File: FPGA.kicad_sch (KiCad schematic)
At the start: 37 parts, among them U7 ICE40HX8K-CB132, X1 XO53

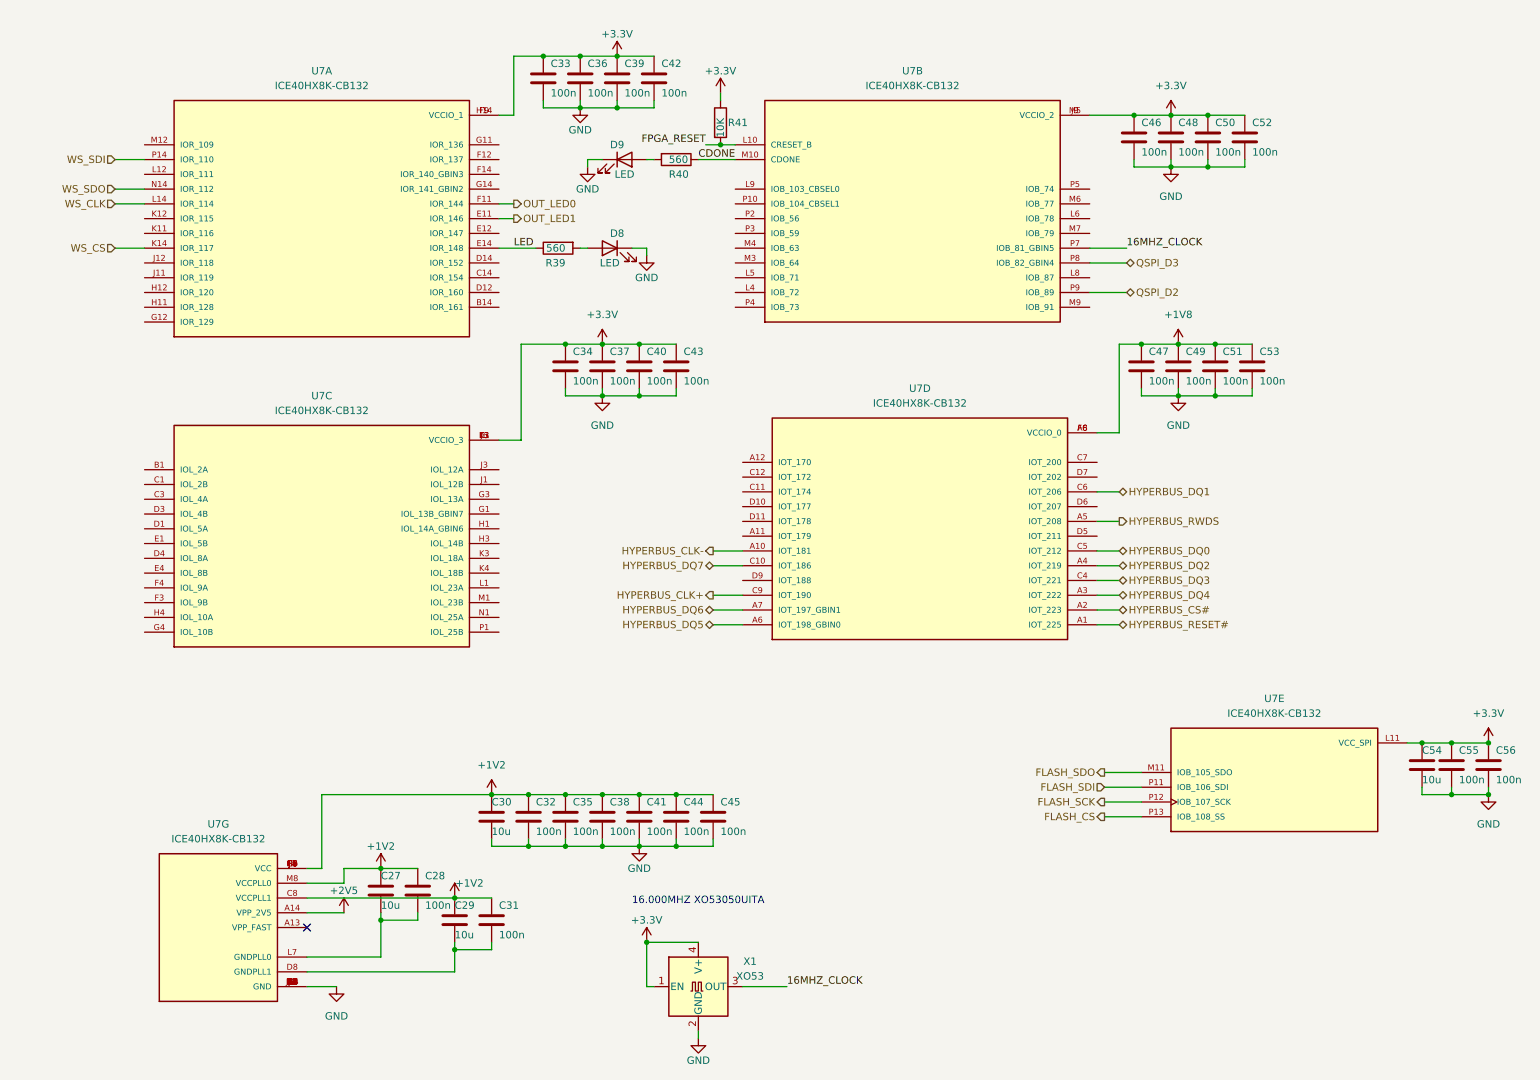
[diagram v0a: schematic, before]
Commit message: Start routing
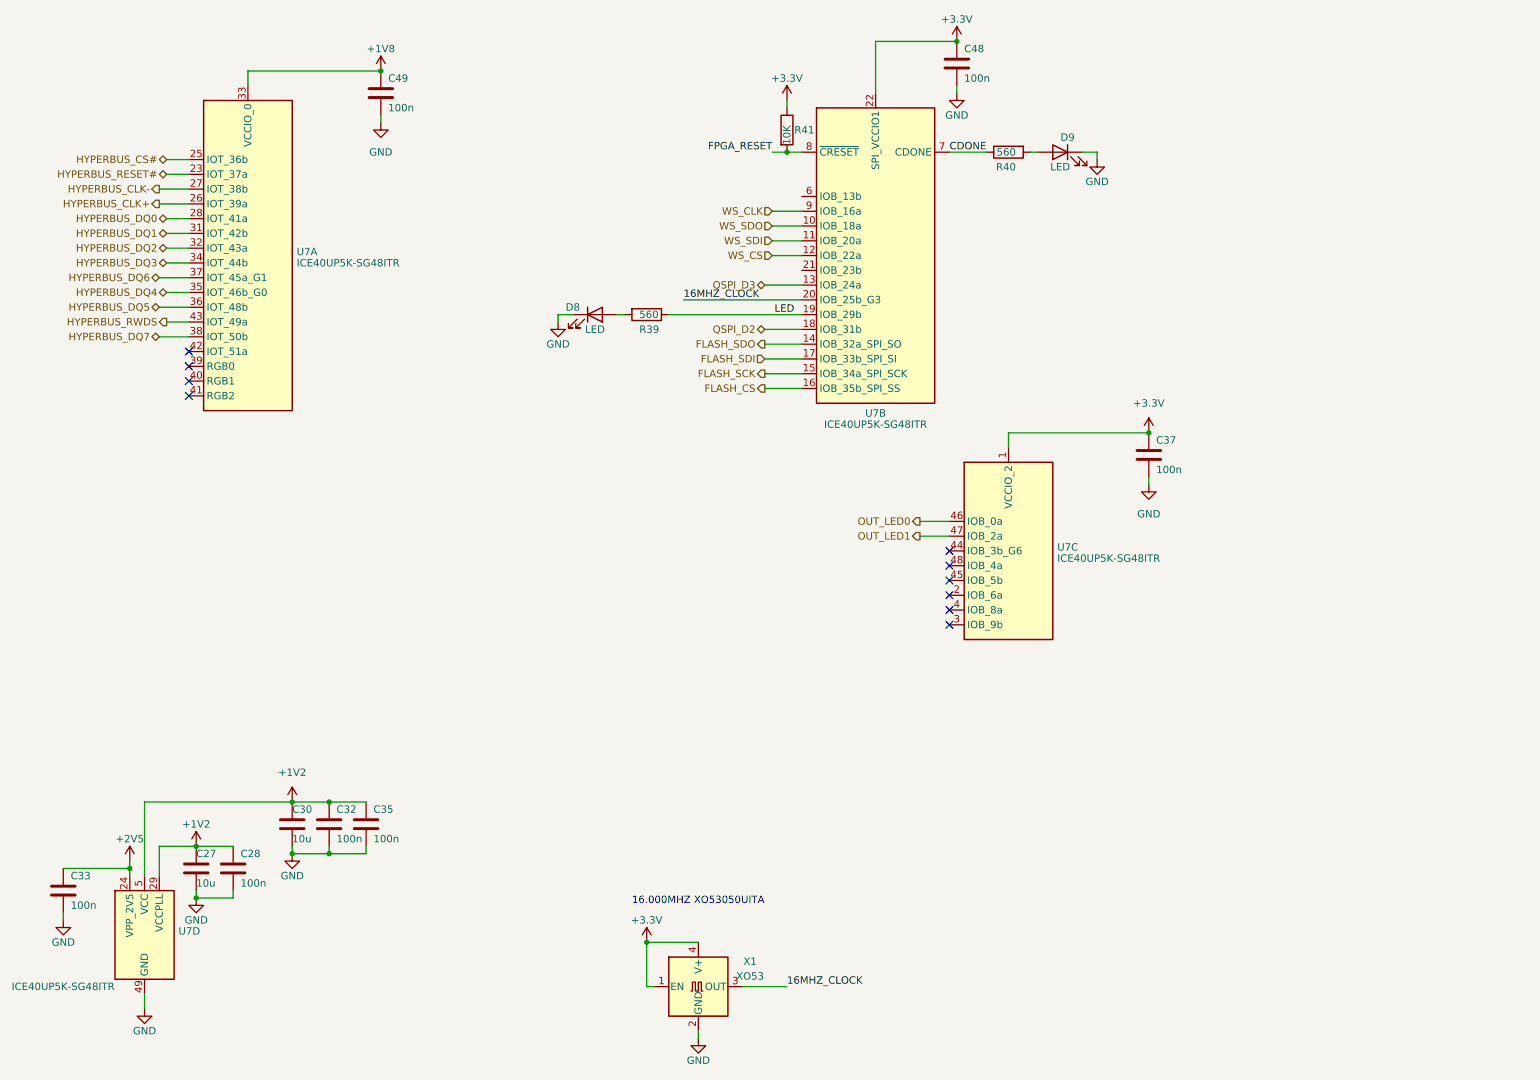
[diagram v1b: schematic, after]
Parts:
- removed C29, C54: 10u, Capacitor_SMD:C_0805_2012Metric, symbol Device:C
- removed C31, C34, C36, C38, C39, C40, C41, C42, C43, C44, C45, C46, C47, C50, C51, C52, C53: 100n, Capacitor_SMD:C_0402_1005Metric, symbol Device:C
- removed C55, C56: 100n, Capacitor_SMD:C_0805_2012Metric, symbol Device:C
- removed U7: ICE40HX8K-CB132, AREA_lib_composant:IC_ICE40HX8K-CB132, symbol AREA_composant:ICE40HX8K-CB132
- added U7: ICE40UP5K-SG48ITR, Package_DFN_QFN:QFN-48-1EP_7x7mm_P0.5mm_EP5.6x5.6mm, symbol FPGA_Lattice:ICE40UP5K-SG48ITR
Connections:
- net +1V2: now also U7.29 (VCCPLL), U7.30 (VCC), U7.5 (VCC)
- net +1V8: now also U7.33 (VCCIO_0)
- net +2V5: now also C33.1, U7.24 (VPP_2V5)
- net +3V3: now also U7.1 (VCCIO_2), U7.22 (SPI_VCCIO1); no longer C33.1
- net 16MHZ_CLOCK: now also U7.20 (IOB_25b_G3)
- net CDONE: now also U7.7 (CDONE)
- net FLASH_CS: now also U7.16 (IOB_35b_SPI_SS)
- net FLASH_SCK: now also U7.15 (IOB_34a_SPI_SCK)
- net FLASH_SDI: now also U7.17 (IOB_33b_SPI_SI)
- net FLASH_SDO: now also U7.14 (IOB_32a_SPI_SO)
- net FPGA_RESET: now also U7.8 (~{CRESET})
- net GND: now also C27.2, C28.2, U7.49 (GND)
- net HYPERBUS_CLK+: now also U7.26 (IOT_39a)
- net HYPERBUS_CLK-: now also U7.27 (IOT_38b)
- net HYPERBUS_CS#: now also U7.25 (IOT_36b)
- net HYPERBUS_DQ0: now also U7.28 (IOT_41a)
- net HYPERBUS_DQ1: now also U7.31 (IOT_42b)
- net HYPERBUS_DQ2: now also U7.32 (IOT_43a)
- net HYPERBUS_DQ3: now also U7.34 (IOT_44b)
- net HYPERBUS_DQ4: now also U7.35 (IOT_46b_G0)
- net HYPERBUS_DQ5: now also U7.36 (IOT_48b)
- net HYPERBUS_DQ6: now also U7.37 (IOT_45a_G1)
- net HYPERBUS_DQ7: now also U7.38 (IOT_50b)
- net HYPERBUS_RESET#: now also U7.23 (IOT_37a)
- net HYPERBUS_RWDS: now also U7.43 (IOT_49a)
- net LED: now also U7.19 (IOB_29b)
- net OUT_LED0: now also U7.46 (IOB_0a)
- net OUT_LED1: now also U7.47 (IOB_2a)
- net QSPI_D2: now also U7.18 (IOB_31b)
- net QSPI_D3: now also U7.13 (IOB_24a)
- net WS_CLK: now also U7.9 (IOB_16a)
- net WS_CS: now also U7.12 (IOB_22a)
- net WS_SDI: now also U7.11 (IOB_20a)
- net WS_SDO: now also U7.10 (IOB_18a)
- no-connect marks 1 -> 10
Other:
- moved on the sheet: C27, C28, C30, C32, C35, C37, C48, C49, D8, D9, R39, R40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
